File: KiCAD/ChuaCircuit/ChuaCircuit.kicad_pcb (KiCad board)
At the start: 2 copper layers, 30 x 50 mm, 23 parts, among them X1 TP3, Y1 TP2

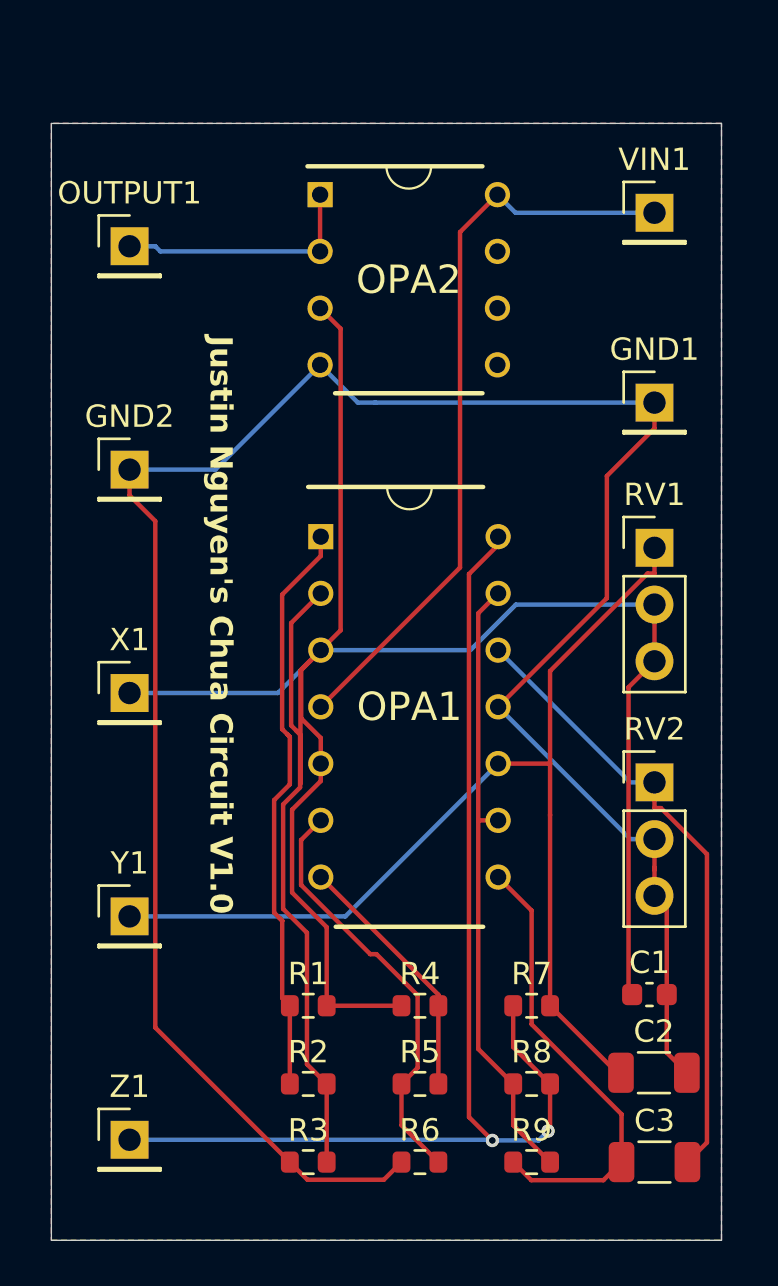
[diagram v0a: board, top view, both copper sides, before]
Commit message: Updated PCB according to new changes
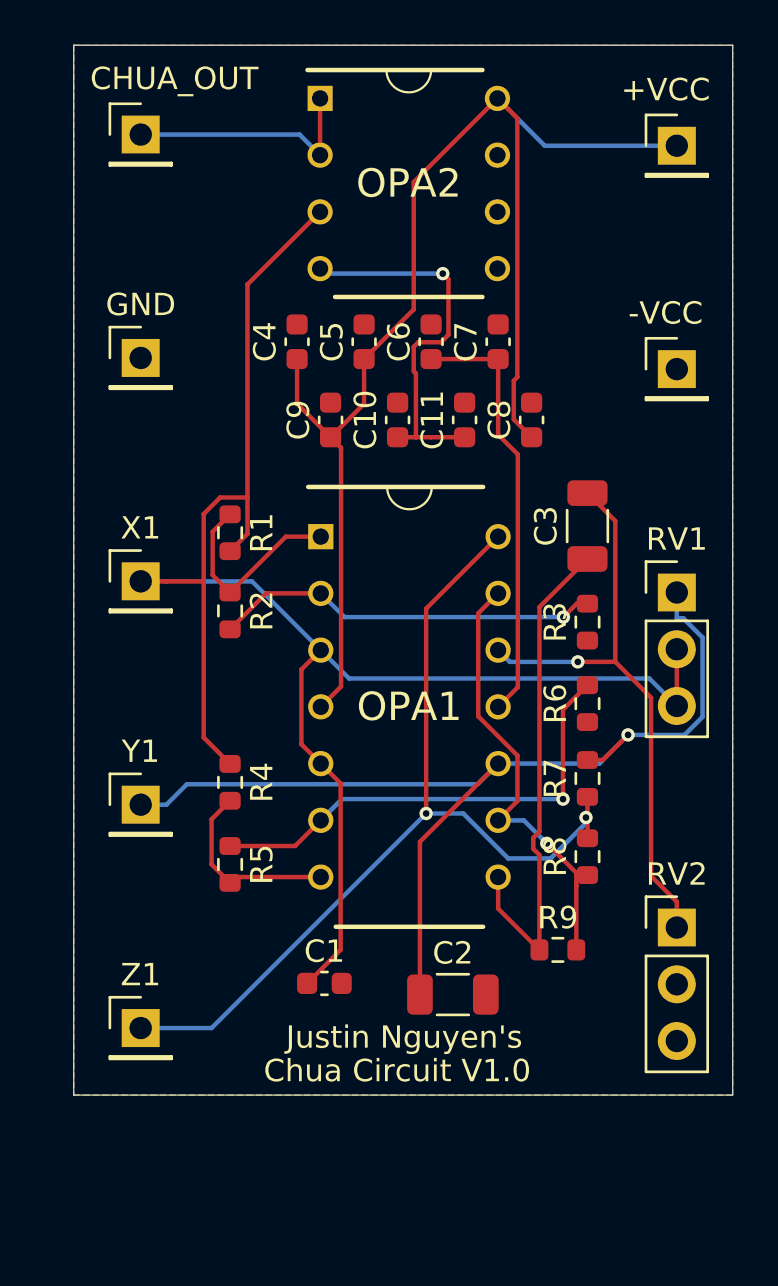
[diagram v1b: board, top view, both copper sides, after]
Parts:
- added C10: 0.1u, Capacitor_SMD:C_0603_1608Metric, F.Cu at (138.0, 89.8)
- added C11: 0.01u, Capacitor_SMD:C_0603_1608Metric, F.Cu at (141.0, 89.8)
- added C4: .01u, Capacitor_SMD:C_0603_1608Metric, F.Cu at (133.5, 86.3)
- added C5: 0.1u, Capacitor_SMD:C_0603_1608Metric, F.Cu at (136.5, 86.3)
- added C6: 0.1u, Capacitor_SMD:C_0603_1608Metric, F.Cu at (139.5, 86.3)
- added C7: 0.01u, Capacitor_SMD:C_0603_1608Metric, F.Cu at (142.5, 86.3)
- added C8: 0.1u, Capacitor_SMD:C_0603_1608Metric, F.Cu at (144.0, 89.8)
- added C9: 0.01u, Capacitor_SMD:C_0603_1608Metric, F.Cu at (135.0, 89.8)
- +VCC: renamed from VIN1; value Male_Header_1x1 -> J1
- -VCC: renamed from GND1; value Male_Header_1x1 -> J1
- moved C3 28.6 mm to (146.5, 94.5), turned to 90 degrees
- moved R3 27.2 mm to (146.5, 98.8), turned to 90 degrees
- moved R6 21.9 mm to (146.5, 102.5), turned to 90 degrees
- moved R1 21.5 mm to (130.5, 94.8), turned to -90 degrees
- moved R2 21.5 mm to (130.5, 98.3), turned to -90 degrees
- moved C1 14.6 mm to (134.7, 115.0)
- moved R4 13.1 mm to (130.5, 106.0), turned to -90 degrees
- moved R5 13.0 mm to (130.5, 109.7), turned to -90 degrees
- moved R7 10.5 mm to (146.5, 105.8), turned to 90 degrees
- moved R8 10.5 mm to (146.5, 109.3), turned to 90 degrees
- moved C2 9.66 mm to (140.5, 115.5)
- moved R9 9.57 mm to (145.2, 113.5)
- moved RV2 6.58 mm to (150.5, 112.5)
- moved CHUA_OUT 5.02 mm to (126.5, 77.0)
- moved GND 5.02 mm to (126.5, 87.0)
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- renumbered OUTPUT1 to CHUA_OUT, GND2 to GND
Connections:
- -VCC pad 1: GND -> Net-(-VCC1-Pin_1)
- OPA1 pad 11: GND -> Net-(-VCC1-Pin_1)
- OPA2 pad 4: GND -> Net-(OPA2C-V-)
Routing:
- net GND: track 102.8 -> 0.00 mm
- net VCC: track 33.6 -> 59.9 mm
- net Net-(-VCC1-Pin_1): track 0.00 -> 19.3 mm
- net Net-(OPA2C-V-): track 0.00 -> 17.3 mm, vias 0 -> 1
- net Net-(OPA1-Pad1): track 26.3 -> 9.24 mm
- net Net-(OPA1-Pad14): track 53.8 -> 41.3 mm
- net Net-(OPA1A--): track 27.5 -> 17.4 mm, vias 0 -> 1
- net Net-(OPA1C--): track 28.0 -> 20.0 mm, vias 0 -> 1
- net Net-(OPA1-Pad7): track 11.4 -> 8.53 mm
- net Net-(OPA1B--): track 19.0 -> 21.3 mm, vias 0 -> 1
- net Net-(C3-Pad1): track 20.6 -> 22.6 mm
- net Net-(OPA1C-+): track 48.7 -> 47.1 mm, vias 0 -> 1
- net Net-(OPA1D-+): track 28.0 -> 26.6 mm, vias 0 -> 1
- net Net-(OPA1A-+): track 80.4 -> 79.1 mm
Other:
- board size 30 x 50 mm -> 29.5 x 47 mm
- board text added: "Chua Circuit V1.0"
- board text added: "Justin Nguyen's"
- board text removed: "Justin Nguyen's Chua Circuit V1.0"
